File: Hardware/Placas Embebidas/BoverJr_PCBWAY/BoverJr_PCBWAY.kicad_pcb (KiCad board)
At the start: 2 copper layers, 100 x 100.1 mm, 55 parts, among them J1 Encoder Derecho, J10 7.4v, J11 Cable_PAD, J2 Encoder Izquierdo, J3 Programador, J4 Distancia_Der, J5 Distancia_Izq, J6 Cable_PAD, J7 Cable_PAD, J8 Distancia_Frontal, J9 Cable_PAD, SW1 SW_SPDT, U1 ESP32-WROOM-32E, U2 MPU, U3 AMS1117-5.0, U5 DRV8833, U7 AMS1117-3.3

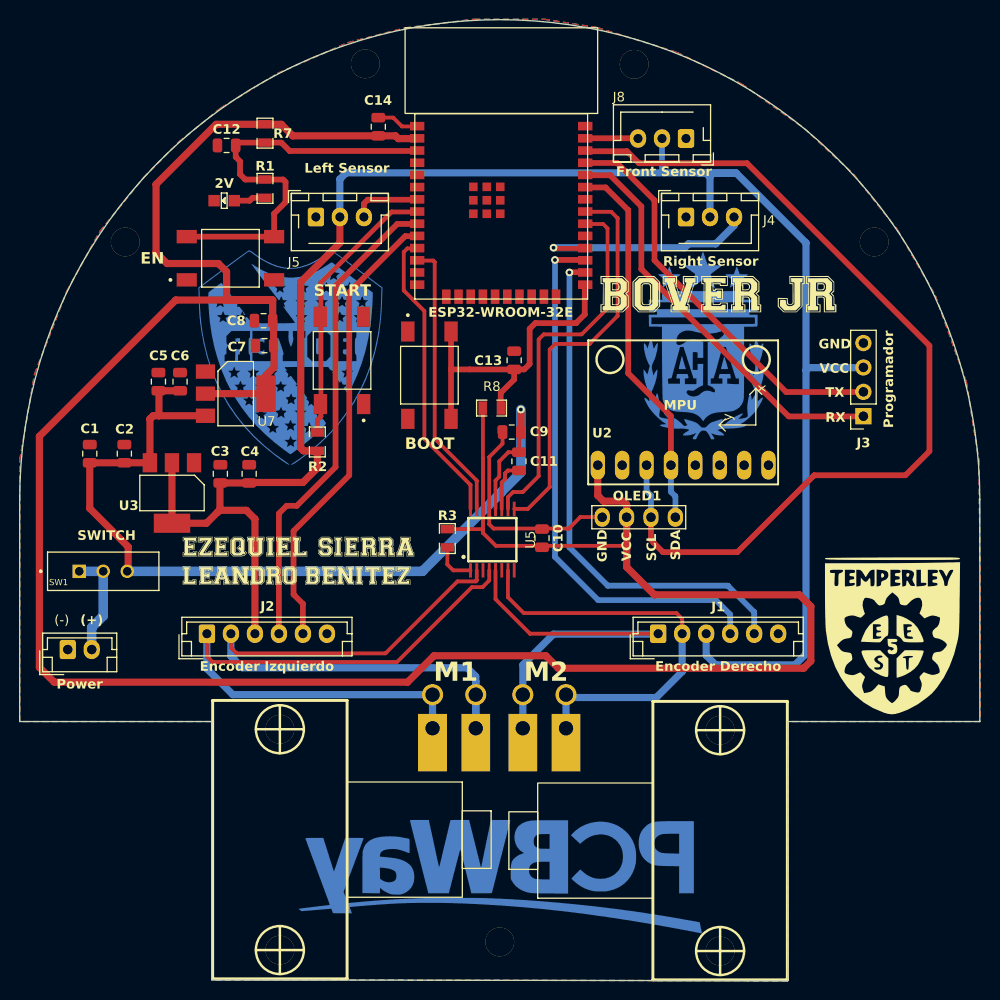
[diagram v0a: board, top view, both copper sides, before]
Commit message: archivos gerber
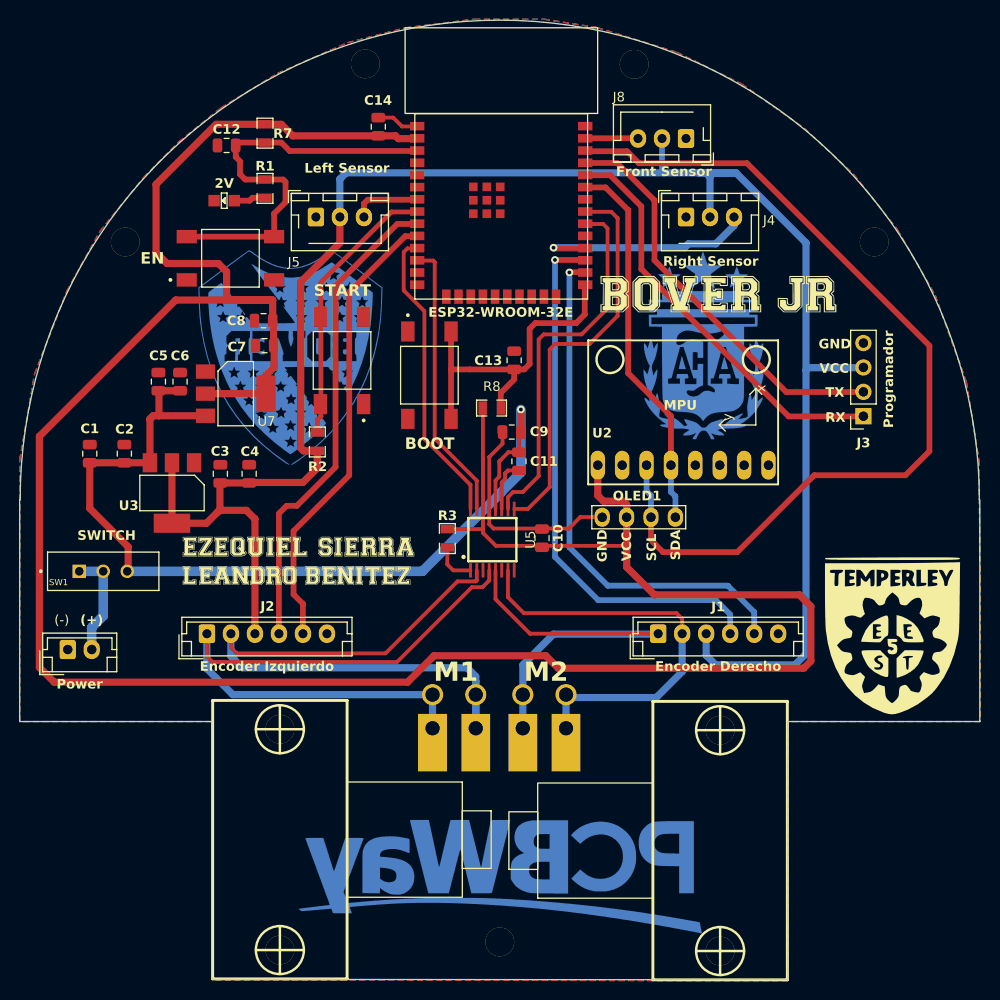
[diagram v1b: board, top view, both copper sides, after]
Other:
- board size 100 x 100.1 mm -> 100 x 100 mm
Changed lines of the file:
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@@
     (pad_to_mask_clearance 0)
     (pcbplotparams
-      (layerselection 0x00010fc_ffffffff)
-      (plot_on_all_layers_selection 0x0000000_00000000)
+      (layerselection 0x00000fc_ffffffff)
+      (plot_on_all_layers_selection 0x0001000_00000000)
       (disableapertmacros false)
       (usegerberextensions false)
       (usegerberattributes true)
       (usegerberadvancedattributes true)
-      (creategerberjobfile true)
+      (creategerberjobfile false)
       (dashed_line_dash_ratio 12.000000)
       (dashed_line_gap_ratio 3.000000)
@@
       (outputformat 1)
       (mirror false)
-      (drillshape 1)
+      (drillshape 0)
       (scaleselection 1)
-      (outputdirectory "")
+      (outputdirectory "Gerber/")
     )
   )
@@
     (fp_line (start 15 2.2) (end 15 -1.6)
       (stroke (width 0.1) (type solid)) (layer "F.Fab"))
-    (pad "1" thru_hole roundrect (at 0 0) (size 1.7 1.95) (drill 0.95) (layers "*.Cu" "*.Mask") (roundrect_rratio 0.147059)
+    (pad "1" thru_hole roundrect (at 0 0) (size 1.7 1.95) (drill 0.95) (layers "*.Cu" "*.Mask") (roundrect_rratio 0.1470588235)
       (net 7 "/OUT_A_MOTOR1") (pinfunction "Pin_1") (pintype "passive"))
     (pad "2" thru_hole oval (at 2.5 0) (size 1.7 1.95) (drill 0.95) (layers "*.Cu" "*.Mask")
@@
     (fp_line (start 5 2.2) (end 5 -1.6)
       (stroke (width 0.1) (type solid)) (layer "F.Fab"))
-    (pad "1" thru_hole roundrect (at 0 0) (size 1.7 2) (drill 1) (layers "*.Cu" "*.Mask") (roundrect_rratio 0.147059)
+    (pad "1" thru_hole roundrect (at 0 0) (size 1.7 2) (drill 1) (layers "*.Cu" "*.Mask") (roundrect_rratio 0.1470588235)
       (net 2 "GND") (pinfunction "Pin_1") (pintype "passive"))
     (pad "2" thru_hole oval (at 2.5 0) (size 1.7 2) (drill 1) (layers "*.Cu" "*.Mask")
@@
     (fp_line (start 7.45 3.4) (end 7.45 -2.35)
       (stroke (width 0.1) (type solid)) (layer "F.Fab"))
-    (pad "1" thru_hole roundrect (at 0 0 180) (size 1.7 1.95) (drill 0.95) (layers "*.Cu" "*.Mask") (roundrect_rratio 0.147059)
+    (pad "1" thru_hole roundrect (at 0 0 180) (size 1.7 1.95) (drill 0.95) (layers "*.Cu" "*.Mask") (roundrect_rratio 0.1470588235)
       (net 2 "GND") (pinfunction "Pin_1") (pintype "passive"))
     (pad "2" thru_hole oval (at 2.5 0 180) (size 1.7 1.95) (drill 0.95) (layers "*.Cu" "*.Mask")
@@
     (fp_line (start 7.45 3.4) (end 7.45 -2.35)
       (stroke (width 0.1) (type solid)) (layer "F.Fab"))
-    (pad "1" thru_hole roundrect (at 0 0) (size 1.7 1.95) (drill 0.95) (layers "*.Cu" "*.Mask") (roundrect_rratio 0.147059)
+    (pad "1" thru_hole roundrect (at 0 0) (size 1.7 1.95) (drill 0.95) (layers "*.Cu" "*.Mask") (roundrect_rratio 0.1470588235)
       (net 2 "GND") (pinfunction "Pin_1") (pintype "passive"))
     (pad "2" thru_hole oval (at 2.5 0) (size 1.7 1.95) (drill 0.95) (layers "*.Cu" "*.Mask")
@@
     (fp_line (start 7.45 3.4) (end 7.45 -2.35)
       (stroke (width 0.1) (type solid)) (layer "F.Fab"))
-    (pad "1" thru_hole roundrect (at 0 0) (size 1.7 1.95) (drill 0.95) (layers "*.Cu" "*.Mask") (roundrect_rratio 0.147059)
+    (pad "1" thru_hole roundrect (at 0 0) (size 1.7 1.95) (drill 0.95) (layers "*.Cu" "*.Mask") (roundrect_rratio 0.1470588235)
       (net 2 "GND") (pinfunction "Pin_1") (pintype "passive"))
     (pad "2" thru_hole oval (at 2.5 0) (size 1.7 1.95) (drill 0.95) (layers "*.Cu" "*.Mask")
@@
     (fp_line (start 15 2.2) (end 15 -1.6)
       (stroke (width 0.1) (type solid)) (layer "F.Fab"))
-    (pad "1" thru_hole roundrect (at 0 0) (size 1.7 1.95) (drill 0.95) (layers "*.Cu" "*.Mask") (roundrect_rratio 0.147059)
+    (pad "1" thru_hole roundrect (at 0 0) (size 1.7 1.95) (drill 0.95) (layers "*.Cu" "*.Mask") (roundrect_rratio 0.1470588235)
       (net 11 "/OUT_A_MOTOR2") (pinfunction "Pin_1") (pintype "passive"))
     (pad "2" thru_hole oval (at 2.5 0) (size 1.7 1.95) (drill 0.95) (layers "*.Cu" "*.Mask")
@@
       (net 11 "/OUT_A_MOTOR2") (pinfunction "1") (pintype "input"))
   )
-  (gr_arc (start 100 79.8) (mid 150 29.8) (end 200 79.8)
+  (gr_arc (start 100.05 79.8) (mid 150 29.85) (end 199.95 79.8)
     (stroke (width 0.1) (type default)) (layer "Edge.Cuts"))
-  (gr_line (start 120 129.8) (end 120 102.9)
+  (gr_line (start 120 129.75) (end 120 102.9)
     (stroke (width 0.1) (type default)) (layer "Edge.Cuts"))
   (gr_line (start 180 102.9) (end 200 102.9)
     (stroke (width 0.1) (type default)) (layer "Edge.Cuts"))
-  (gr_line (start 180 129.9) (end 180 102.9)
+  (gr_line (start 180 129.85) (end 180 102.9)
     (stroke (width 0.1) (type default)) (layer "Edge.Cuts"))
   (gr_line (start 120 102.9) (end 100 102.9)
@@
   (gr_line (start 200 102.9) (end 200 79.8)
     (stroke (width 0.1) (type default)) (layer "Edge.Cuts"))
-  (gr_line (start 120 129.8) (end 180 129.9)
+  (gr_line (start 120 129.75) (end 180 129.8)
     (stroke (width 0.1) (type default)) (layer "Edge.Cuts"))
   (gr_text "(-)" (at 103.6 92.9) (layer "F.SilkS")
@@
   )
   (dimension (type aligned) (layer "Dwgs.User")
-    (pts (xy 200 102.9) (xy 100 102.9))
+    (pts (xy 200.05 102.9) (xy 99.95 102.9))
     (height -41.05)
-    (gr_text "100,0000 mm" (at 150 142.8) (layer "Dwgs.User")
+    (gr_text "100,1000 mm" (at 150 142.8) (layer "Dwgs.User")
       (effects (font (size 1 1) (thickness 0.15)))
     )
@@
   )
   (dimension (type aligned) (layer "Dwgs.User")
-    (pts (xy 150 29.8) (xy 150.1 129.8))
+    (pts (xy 150 29.8) (xy 150.1 129.9))
     (height 56.709466)
-    (gr_text "100,0000 mm" (at 94.490561 79.855559 270.0572958) (layer "Dwgs.User")
+    (gr_text "100,1000 mm" (at 94.490561 79.905504 270.0572385) (layer "Dwgs.User")
       (effects (font (size 1 1) (thickness 0.15)))
     )
